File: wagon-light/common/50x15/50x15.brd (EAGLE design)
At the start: 116 x 12 mm, 32 parts, among them IC2 78L05F, IC3 16F18324-SL, Q1 BC817-25SMD, U1 BCR421U, U2 BCR421U, U3 BCR421U

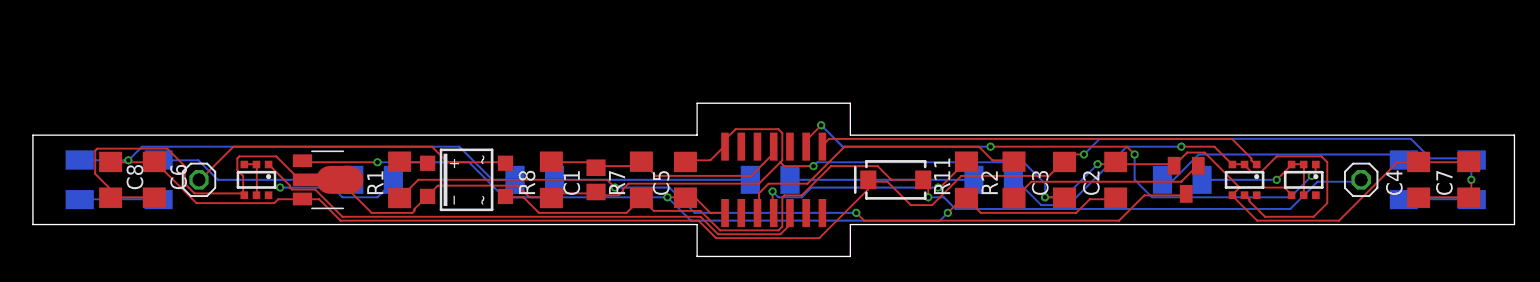
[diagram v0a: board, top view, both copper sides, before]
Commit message: misc
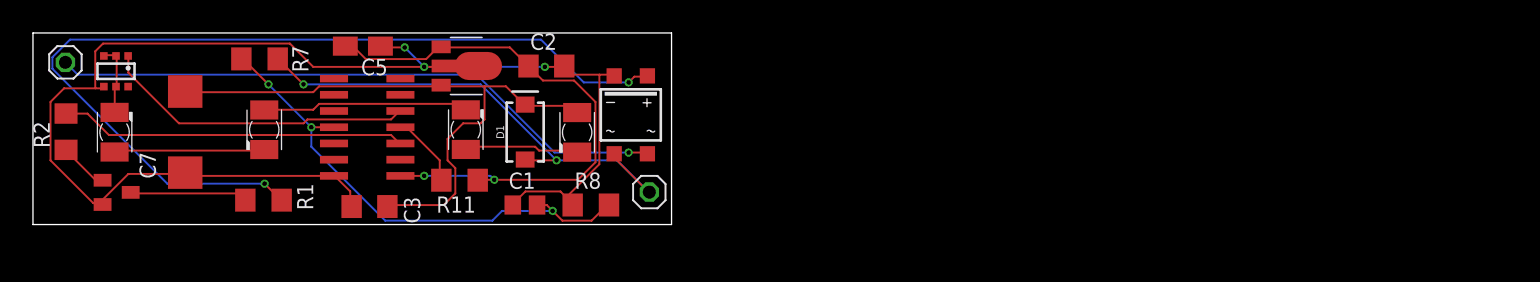
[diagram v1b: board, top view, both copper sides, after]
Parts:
- removed C4, C6, C8: 10u/35V, rcl:C3216
- removed LED10, LED11, LED5, LED6, LED7, LED9: (no value), led:KA-3528ASYC
- removed U2, U3: BCR421U, BCR421U:SC74-6
- added LED4: (no value), led:KA-3528ASYC
- C5: device rcl:C3216 -> rcl:A/3216-18R
- C7: device rcl:C3216 -> rcl:D/7343-31R
- moved C7 100.6 mm to (11.9, 7.24)
- moved Q1 83.8 mm to (6.55, 2.52), turned to 270 degrees
- moved R2 74.3 mm to (2.59, 7.27)
- moved JP3 55.7 mm to (48.3, 2.54)
- moved C3 54.5 mm to (26.4, 1.41), turned to 0 degrees
- moved C2 45.5 mm to (40.2, 12.4), turned to 0 degrees
- moved R11 39.7 mm to (33.4, 3.47), turned to 180 degrees
- moved LED1 39.1 mm to (42.6, 7.22), flipped to the top
- moved IC3 32.1 mm to (26.2, 7.62), turned to 90 degrees
- moved R7 31.4 mm to (17.7, 13.0), turned to 180 degrees
- moved D1 29.3 mm to (38.5, 7.24), turned to 90 degrees
- moved C5 27.3 mm to (25.8, 14.0), turned to 180 degrees
- moved LED2 24.4 mm to (33.9, 7.43), flipped to the top
- moved IC2 14.0 mm to (33.9, 12.4)
- moved JP4 13.9 mm to (2.54, 12.7)
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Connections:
- net PWM1 renamed N$6
- removed net N$16: LED10.C, LED11.A
- removed net N$19: LED6.C, LED7.A
- removed net N$22: LED5.C, LED6.A
- removed net N$23: LED10.A, LED9.C
- removed net N$30: LED3.C, U1.2, U1.3, U1.5
- removed net N$31: LED11.C, U3.2, U3.3, U3.5
- removed net N$32: LED7.C, U2.2, U2.3, U2.5
- removed net PWM2: IC3.9, U2.1
- removed net PWM3: IC3.8, U3.1
- removed net PWM4: IC3.7
- removed net PWM6: IC3.10
- new net N$10: LED3.C, LED4.A
- new net N$8: LED4.C, U1.2, U1.3, U1.5
- net +15V: now also C7.+; no longer C4.1, C6.1, C7.1, C8.1, LED5.A, LED9.A
- net +5V: now also C5.+; no longer C5.1
- net GND: now also C5.-, C7.-; no longer C4.2, C5.2, C6.2, C7.2, C8.2, U2.4, U3.4
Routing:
- net +15V: track 158.2 -> 48.2 mm, vias 3 -> 0
- net N$5: track 2.22 -> 71.9 mm, vias 0 -> 2
- net N$3: track 64.4 -> 9.25 mm, vias 2 -> 0
- net PWM2: track 45.8 -> 0.00 mm, vias 4 -> 0
- net GND: track 152.3 -> 108.0 mm
- net N$31: track 39.8 -> 0.00 mm, vias 1 -> 0
- net N$2: track 75.4 -> 40.1 mm, vias 1 -> 2
- net PWM3: track 35.2 -> 0.00 mm
- net +5V: track 72.4 -> 44.3 mm, vias 3 -> 2
- net N$1: track 25.6 -> 48.5 mm, vias 0 -> 1
- net N$19: track 19.9 -> 0.00 mm
- net N$6: track 44.4 -> 24.6 mm
- net COMMAND: track 19.6 -> 39.2 mm, vias 0 -> 3
- net N$23: track 15.3 -> 0.00 mm
- net N$30: track 15.0 -> 0.00 mm, vias 1 -> 0
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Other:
- board size 116 x 12 mm -> 50 x 15 mm
- board text removed: "https://github.com/stb49078/nscale-adapter-decoder"
